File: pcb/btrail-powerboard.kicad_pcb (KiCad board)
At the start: 2 copper layers, 64.1 x 61.3 mm, 13 parts, among them J1 RJ45 Shielded, Q1 IRLZ34N

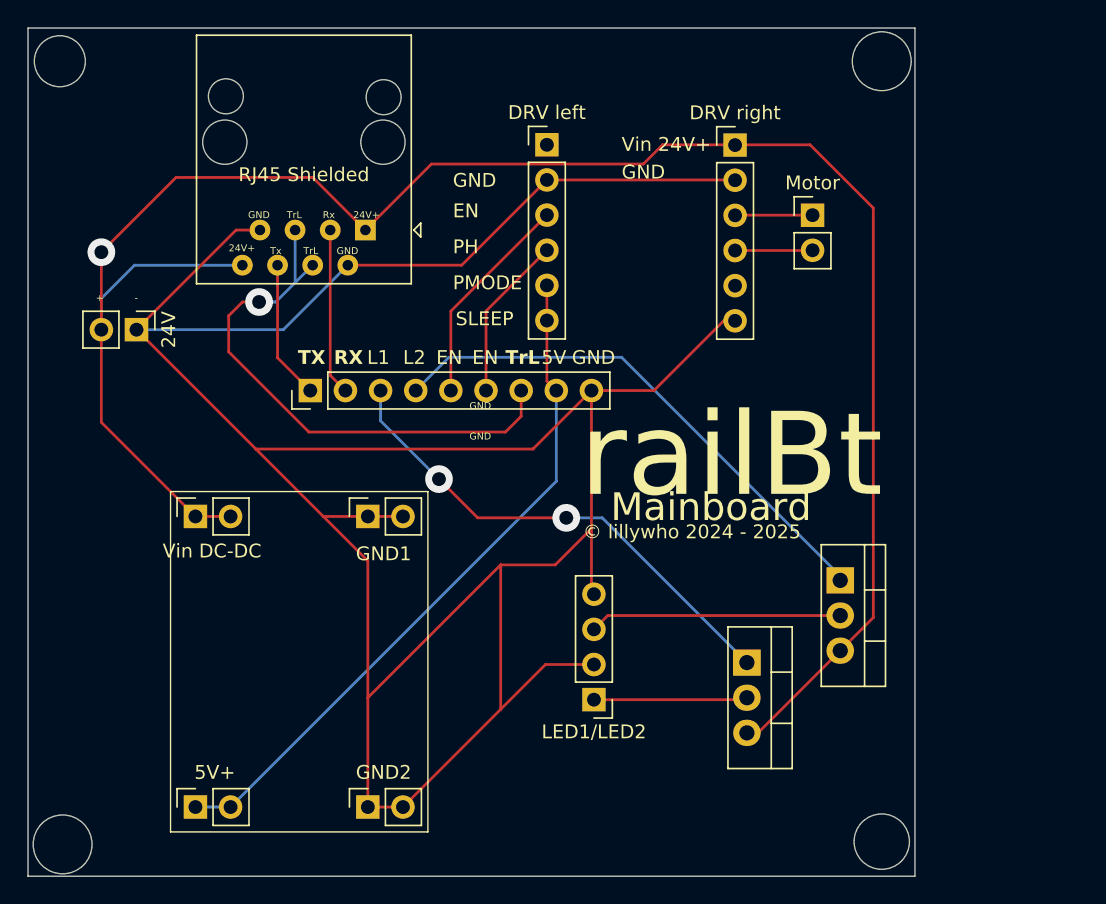
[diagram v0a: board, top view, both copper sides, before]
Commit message: Final revision, added ground plane and more compact design, thanks Emily!
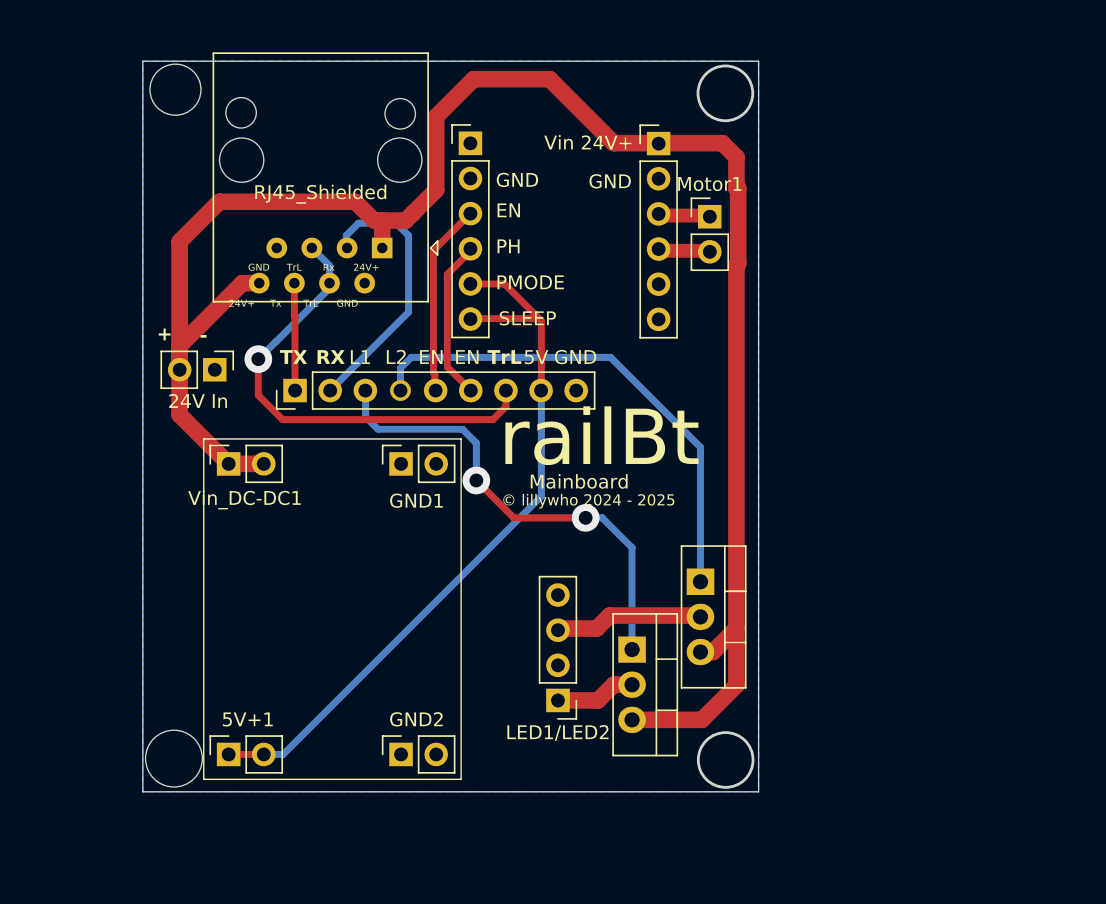
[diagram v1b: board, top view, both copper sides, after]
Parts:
- removed 24V, Motor: Conn_01x02_Pin, Connector_PinHeader_2.54mm:PinHeader_1x02_P2.54mm_Vertical
- added 24V In: Conn_01x02_Pin, Connector_PinHeader_2.54mm:PinHeader_1x02_P2.54mm_Vertical, F.Cu at (195.4, 40.7)
- added Motor1: Conn_01x02_Pin, Connector_PinHeader_2.54mm:PinHeader_1x02_P2.54mm_Vertical, F.Cu at (231.2, 29.6)
- DRV8874_left1: renamed from DRV left
- DRV8874_right1: renamed from DRV right
- J1: value RJ45 Shielded -> RJ45_Shielded
- Vin_DC-DC1: renamed from Vin DC-DC
- moved Q1 10.1 mm to (230.5, 56.0)
- moved Q2 8.35 mm to (225.6, 60.9)
- moved DRV8874_left1 5.53 mm to (213.9, 24.3)
- moved DRV8874_right1 5.53 mm to (227.5, 24.4)
- moved 5V+1 4.49 mm to (196.4, 68.5)
- moved GND1 4.49 mm to (208.9, 47.5)
- moved GND2 4.49 mm to (208.9, 68.5)
- moved Vin_DC-DC1 4.49 mm to (196.4, 47.5)
- moved LED1/LED2 2.60 mm to (220.2, 64.6)
- moved J1 1.78 mm to (207.5, 31.9)
- moved ESP32_jack1 1.10 mm to (201.2, 42.2)
- renumbered 5V+ to 5V+1, IRLZ34N to Q2
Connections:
- net Net-(5V+1-Pin_1) renamed +5V
- net Net-(DRV_left1-Pin_2) renamed GND
- net Net-(DRV_right1-Pin_1) renamed +24V
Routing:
- net GND: track 212.4 -> 0.00 mm
- net +24V: track 144.1 -> 133.3 mm, vias 1 -> 0
- net Net-(ESP32_jack1-Pin_2): track 12.1 -> 19.7 mm
- net Net-(LED1/LED2-Pin_3): track 18.2 -> 10.8 mm
- net Net-(ESP32_jack1-Pin_7): track 39.9 -> 33.5 mm
- net Net-(LED1/LED2-Pin_1): track 10.7 -> 5.83 mm
- net +5V: track 50.3 -> 54.2 mm
- net Net-(ESP32_jack1-Pin_4): track 38.5 -> 36.0 mm
- net Net-(ESP32_jack1-Pin_1): track 10.0 -> 7.78 mm
- net Net-(DRV8874_right1-Pin_4): track 5.61 -> 3.58 mm
- net Net-(DRV8874_right1-Pin_3): track 5.61 -> 3.58 mm
- net Net-(ESP32_jack1-Pin_3): track 35.9 -> 34.0 mm
- net Net-(DRV8874_left1-Pin_3): track 15.6 -> 13.9 mm
- added copper zone on B.Cu, net GND
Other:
- board size 64.1 x 61.3 mm -> 44.5 x 52.8 mm
